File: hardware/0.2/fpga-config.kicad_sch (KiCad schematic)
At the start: 30 parts, among them J2 JTAG, J5 USB_Type_C_2.0, Q500 BSS138, SW1 PTS810, U1 W25Q128JVPIQ, U2 ECP5U_12_CABGA256, U6 USBLC6-2P6

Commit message: bom fix
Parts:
- C516, C521, C522, C523: MPN CC0402KRX7R7BB103 -> CC0402KRX7R7BB104
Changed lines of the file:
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@@
   (junction (at 247.65 63.5) (diameter 1.016) (color 0 0 0 0))
   (junction (at 247.65 77.47) (diameter 1.016) (color 0 0 0 0))
+  (no_connect (at 208.28 128.27))
   (no_connect (at 208.28 151.13))
+  (no_connect (at 52.07 80.01))
+  (no_connect (at 208.28 125.73))
+  (no_connect (at 208.28 118.11))
   (no_connect (at 208.28 148.59))
   (no_connect (at 52.07 82.55))
-  (no_connect (at 208.28 125.73))
-  (no_connect (at 52.07 80.01))
-  (no_connect (at 208.28 118.11))
   (no_connect (at 208.28 123.19))
   (no_connect (at 208.28 143.51))
-  (no_connect (at 208.28 128.27))
   (bus_entry (at 120.65 66.04) (size 2.54 -2.54)
     (stroke (width 0.1524) (type solid) (color 0 0 0 0))
@@
       (effects (font (size 1.27 1.27)) (justify left))
     )
-    (property "MPN" "CC0402KRX7R7BB103" (id 5) (at 146.05 158.75 0)
+    (property "MPN" "CC0402KRX7R7BB104" (id 5) (at 146.05 158.75 0)
       (effects (font (size 1.27 1.27)) hide)
     )
@@
       (effects (font (size 1.27 1.27)) (justify left))
     )
-    (property "MPN" "CC0402KRX7R7BB103" (id 5) (at 168.91 158.75 0)
+    (property "MPN" "CC0402KRX7R7BB104" (id 5) (at 168.91 158.75 0)
       (effects (font (size 1.27 1.27)) hide)
     )
@@
       (effects (font (size 1.27 1.27)) hide)
     )
-    (property "MPN" "CC0402KRX7R7BB103" (id 5) (at 185.42 92.71 0)
+    (property "MPN" "CC0402KRX7R7BB104" (id 5) (at 185.42 92.71 0)
       (effects (font (size 1.27 1.27)) hide)
     )
@@
       (effects (font (size 1.27 1.27)) hide)
     )
-    (property "MPN" "CC0402KRX7R7BB103" (id 5) (at 252.73 68.58 0)
-      (effects (font (size 1.27 1.27)) hide)
-    )
+    (property "MPN" "CC0402KRX7R7BB104" (id 5) (at 252.73 68.58 0)
+      (effects (font (size 1.27 1.27)) hide)
+    )

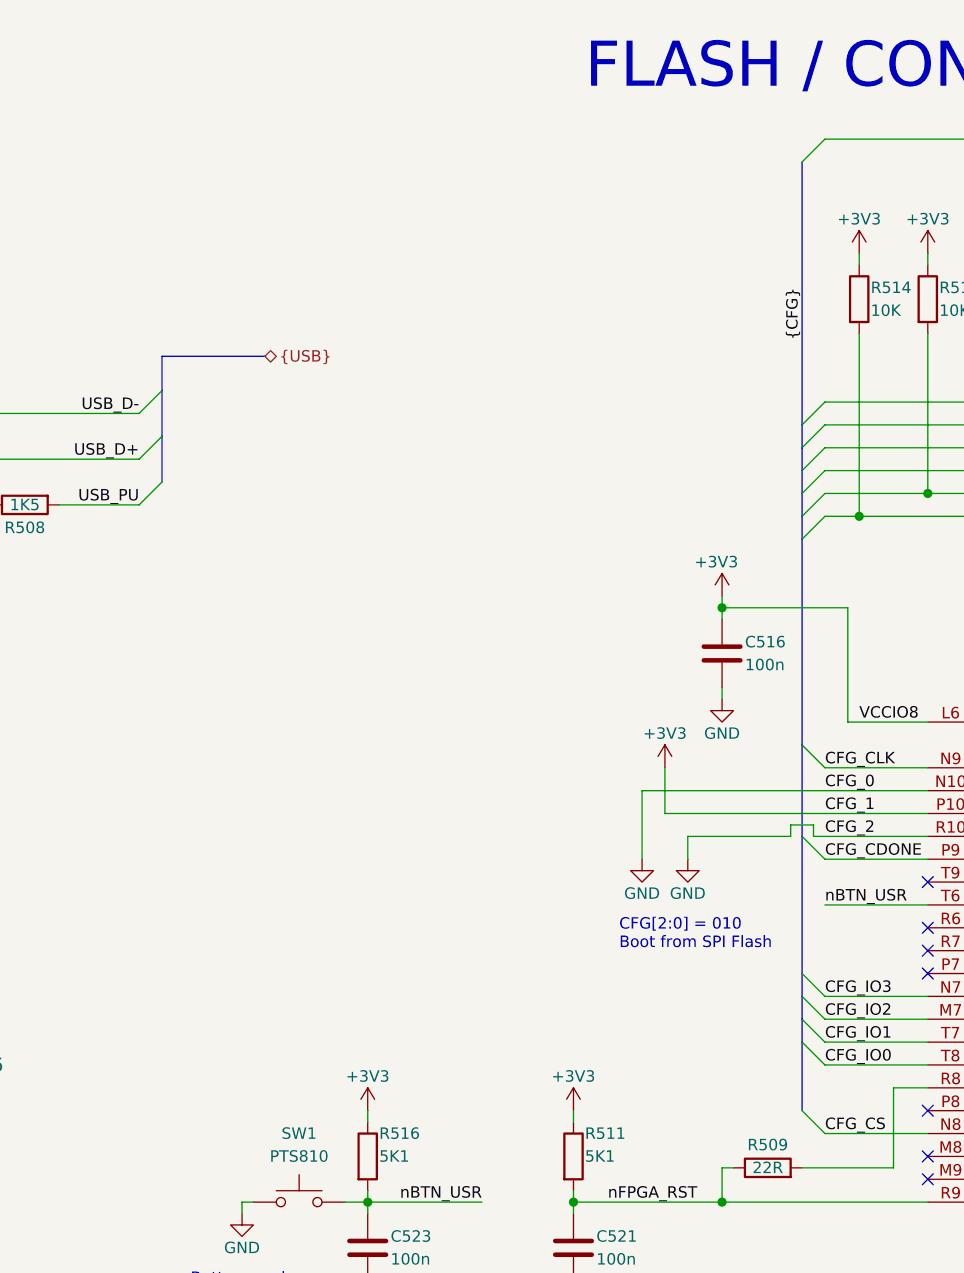
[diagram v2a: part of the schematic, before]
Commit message: nightly version bump
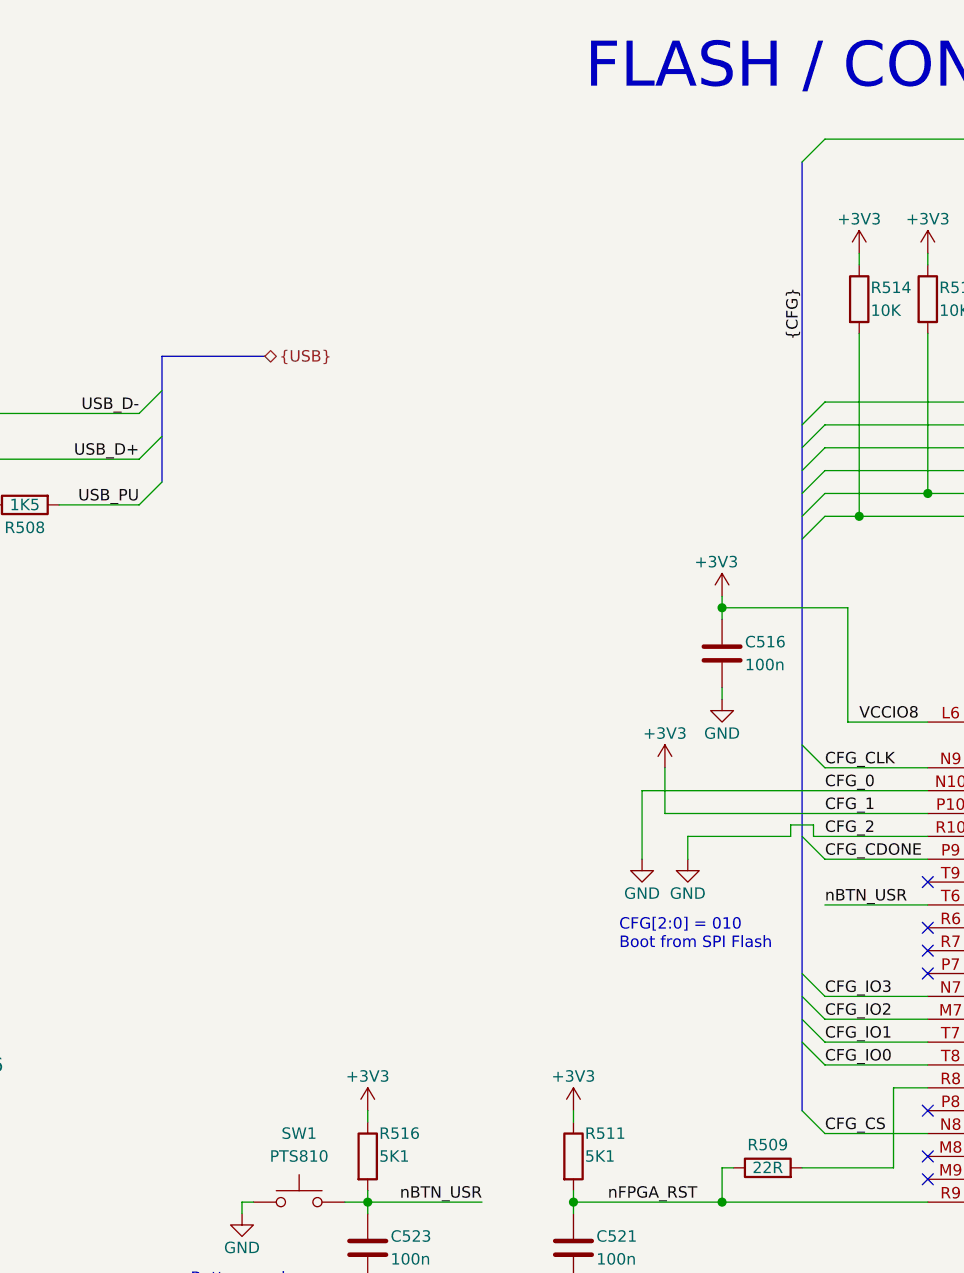
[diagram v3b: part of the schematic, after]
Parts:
- C16: MPN2 CL05A475KP5NRNC -> (none)
- C516, C522: MPN2 CL05B104KO5NNNC -> (none)
- C521, C523: LCSC C327009 -> (none); MPN2 CL05B104KO5NNNC -> (none)
- F1: MPN2 JK-SMD0603-100L -> (none)
- J5: MPN2 TYPE-C-31-M-12 -> (none)
- Q500: MPN2 BSS138W-7-F -> (none)
- R501, R508: MPN2 0402WGF1501TCE -> (none)
- R504, R505: MPN2 0402WGF5101TCE -> (none)
- R506, R507: MPN2 0402WGJ0220TCE -> (none)
- R509: LCSC C93929 -> (none); MPN2 0402WGJ0220TCE -> (none)
- R511, R516: LCSC C105873 -> (none); MPN2 0402WGF5101TCE -> (none)
- R512, R514, R517, R518, R519: MPN2 0402WGJ0103TCE -> (none)
- SW1: MPN2 SKRPACE010 -> (none)
